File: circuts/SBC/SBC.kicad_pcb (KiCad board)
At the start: 2 copper layers, 141 parts, among them IC1 PIC16F15243-I_SS, J1 DE9_Plug, J10 Power, J2 OSTTC060162, J3 XT60-M, J4 OSTTC060162, J5 640456-3, J8 B5B-XH-A_LF__SN_, Q1 IRFS4227, Q10 MMBTA06, Q2 MMBTA06, Q3 MMBTA06, Q4 MMBTA06, Q5 MMBTA06, Q8 IRFS4227, Q9 MMBTA06, U1 3.3v, U2 UC3843, U3 BTS7960B, U5 LM358DT, U6 BTS7960B, U7 BTS7960B, U8 BTS7960B, U9 LM358DT

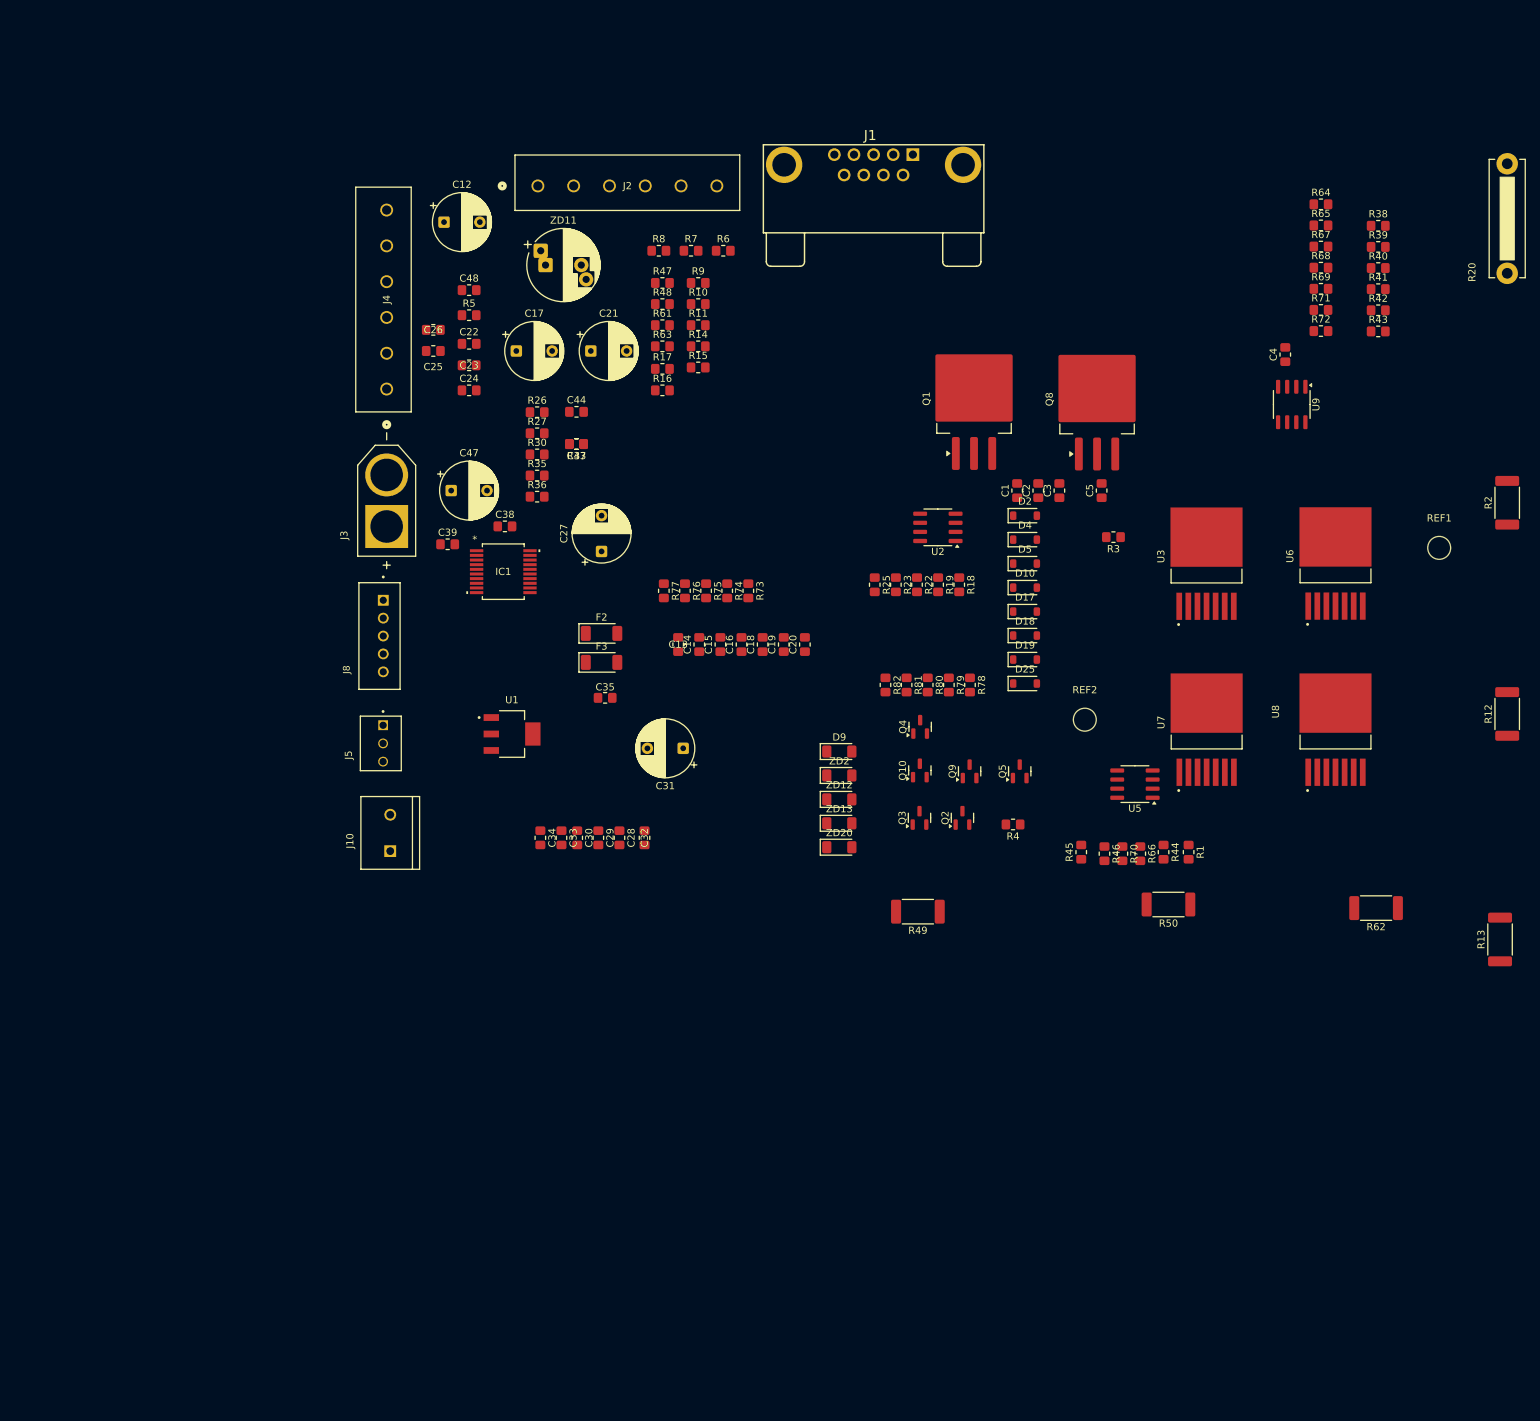
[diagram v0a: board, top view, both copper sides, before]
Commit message: layout
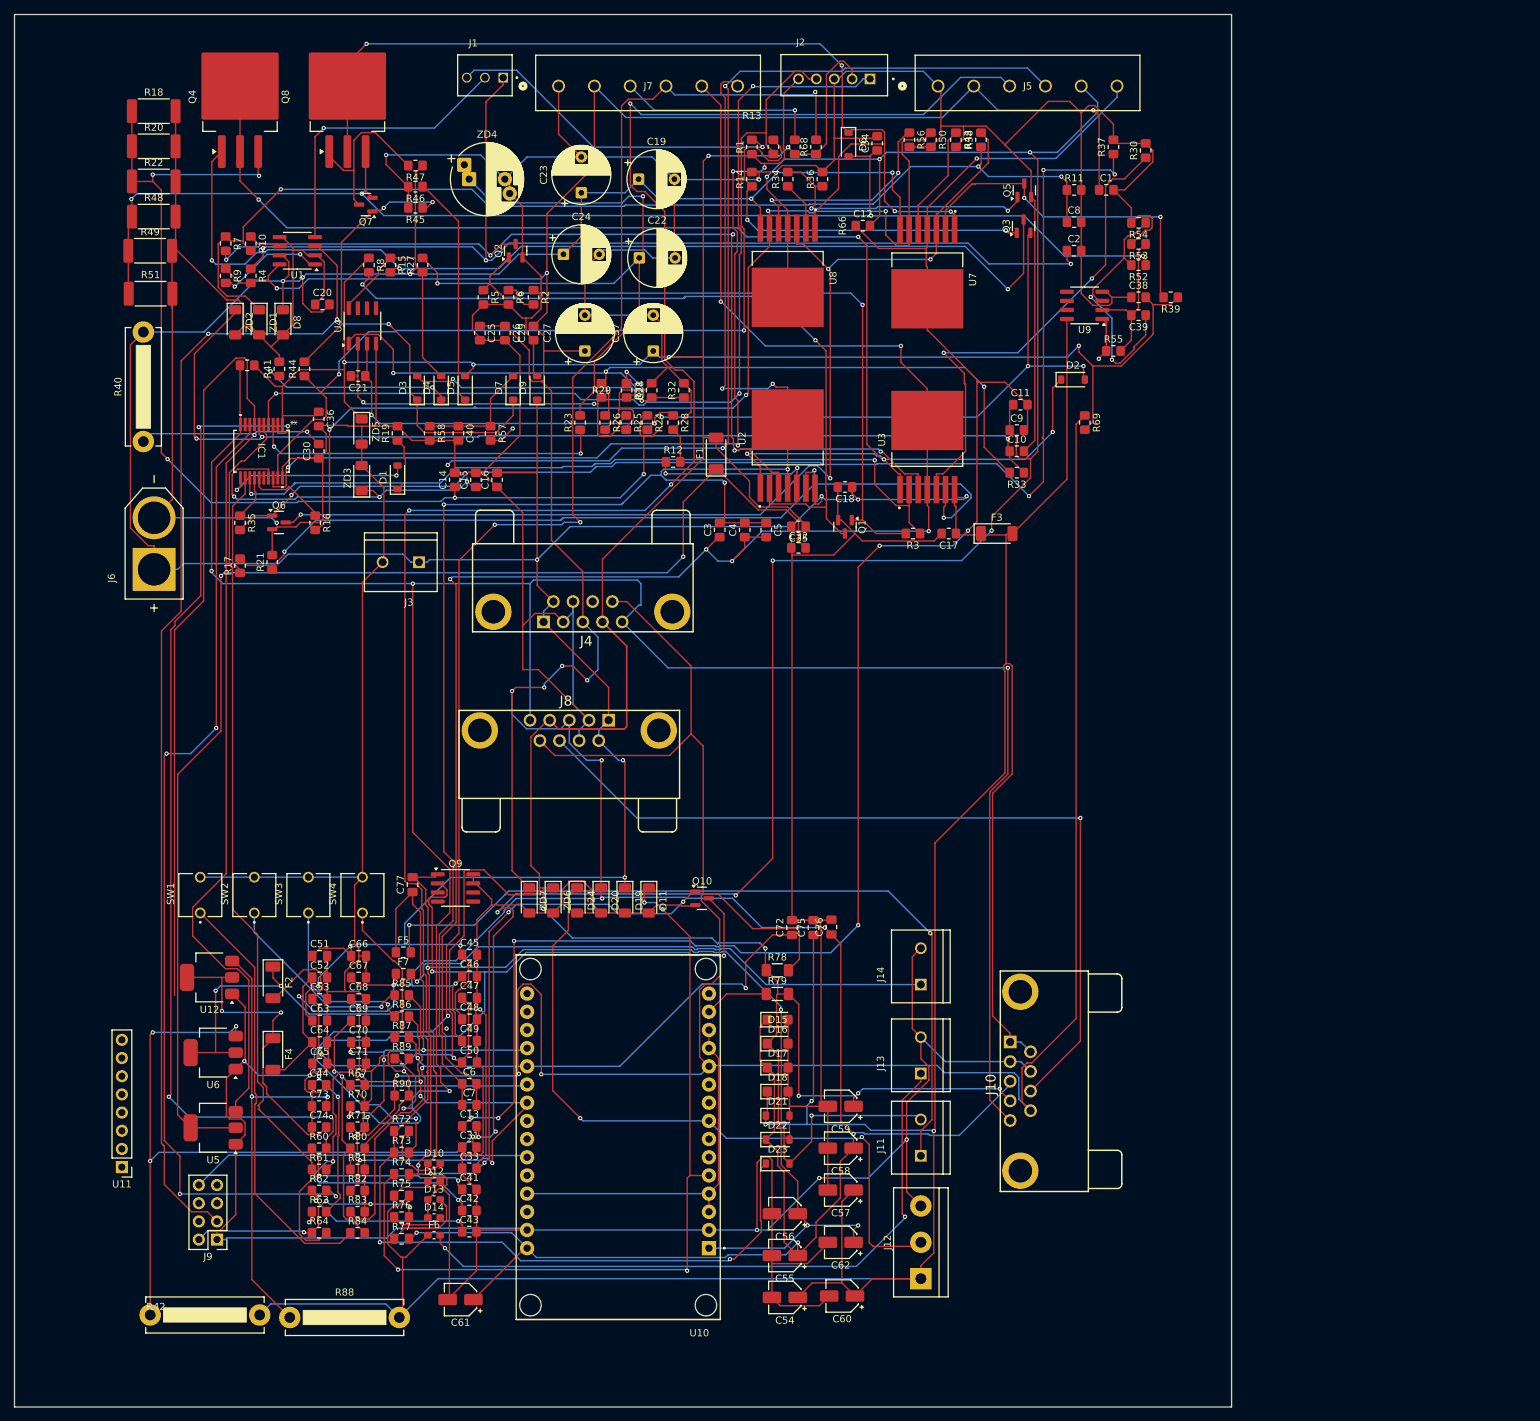
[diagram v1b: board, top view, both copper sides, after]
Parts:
- removed D25: 1N4004-T_NRND, Diode_SMD:D_SOD-123
- removed REF1, REF2: MountingHole_3.2mm_M3, MountingHole:MountingHole_3.2mm_M3
- removed ZD11: BZV55B4V7, Capacitor_THT:CP_Radial_D10.0mm_P5.00mm_P7.50mm
- removed ZD12, ZD13: BZV55B4V7, Diode_SMD:D_MiniMELF
- removed ZD20: 3.3v, Diode_SMD:D_MiniMELF
- added C10: 2uf, Resistor_SMD:R_0805_2012Metric_Pad1.20x1.40mm_HandSolder, F.Cu at (149.0, 77.0)
- added C11: 1nf, Resistor_SMD:R_0805_2012Metric_Pad1.20x1.40mm_HandSolder, F.Cu at (149.5, 70.5)
- added C36: 1nf, Resistor_SMD:R_0805_2012Metric_Pad1.20x1.40mm_HandSolder, F.Cu at (51.5, 72.5)
- added C37: 470uf, Capacitor_THT:CP_Radial_D8.0mm_P5.00mm, F.Cu at (98.2, 63.0)
- added C40: 2uf, Resistor_SMD:R_0805_2012Metric_Pad1.20x1.40mm_HandSolder, F.Cu at (71.0, 74.5)
- added C41: 1nf, Resistor_SMD:R_0805_2012Metric_Pad1.20x1.40mm_HandSolder, F.Cu at (72.5, 180.1)
- added C42: 1nf, Resistor_SMD:R_0805_2012Metric_Pad1.20x1.40mm_HandSolder, F.Cu at (72.5, 183.1)
- added C45: 1nf, Capacitor_SMD:C_0805_2012Metric_Pad1.18x1.45mm_HandSolder, F.Cu at (72.6, 147.3)
- added C46: 1nf, Capacitor_SMD:C_0805_2012Metric_Pad1.18x1.45mm_HandSolder, F.Cu at (72.6, 150.3)
- added C49: 100nf, Capacitor_SMD:C_0805_2012Metric_Pad1.18x1.45mm_HandSolder, F.Cu at (72.6, 159.4)
- added C50: 100nf, Capacitor_SMD:C_0805_2012Metric_Pad1.18x1.45mm_HandSolder, F.Cu at (72.6, 162.4)
- added C51: 2uf, Capacitor_SMD:C_0805_2012Metric_Pad1.18x1.45mm_HandSolder, F.Cu at (51.6, 147.5)
- added C52: 2uf, Capacitor_SMD:C_0805_2012Metric_Pad1.18x1.45mm_HandSolder, F.Cu at (51.6, 150.5)
- added C53: 2uf, Capacitor_SMD:C_0805_2012Metric_Pad1.18x1.45mm_HandSolder, F.Cu at (51.6, 153.5)
- added C54: 100uf, Capacitor_SMD:CP_Elec_4x4.5, F.Cu at (116.6, 195.2)
- added C55: 100uf, Capacitor_SMD:CP_Elec_4x4.5, F.Cu at (116.6, 189.3)
- added C56: 100uf, Capacitor_SMD:CP_Elec_4x4.5, F.Cu at (116.6, 183.5)
- added C57: 470uf, Capacitor_SMD:CP_Elec_4x4.5, F.Cu at (124.4, 180.2)
- added C58: 470uf, Capacitor_SMD:CP_Elec_4x4.5, F.Cu at (124.4, 174.3)
- added C59: 470uf, Capacitor_SMD:CP_Elec_4x4.5, F.Cu at (124.4, 168.5)
- added C6: 2uf, Resistor_SMD:R_0805_2012Metric_Pad1.20x1.40mm_HandSolder, F.Cu at (72.5, 165.4)
- added C60: 1000uf, Capacitor_SMD:CP_Elec_4x4.5, F.Cu at (124.6, 195.0)
- added C61: 1000uf, Capacitor_SMD:CP_Elec_4x4.5, F.Cu at (71.3, 195.5)
- added C62: 1000uf, Capacitor_SMD:CP_Elec_4x4.5, F.Cu at (124.4, 187.5)
- added C63: 2uf, Capacitor_SMD:C_0805_2012Metric_Pad1.18x1.45mm_HandSolder, F.Cu at (51.6, 156.5)
- added C64: 2uf, Capacitor_SMD:C_0805_2012Metric_Pad1.18x1.45mm_HandSolder, F.Cu at (51.6, 159.5)
- added C65: 2uf, Capacitor_SMD:C_0805_2012Metric_Pad1.18x1.45mm_HandSolder, F.Cu at (51.6, 162.5)
- added C66: 100nf, Capacitor_SMD:C_0805_2012Metric_Pad1.18x1.45mm_HandSolder, F.Cu at (57.1, 147.5)
- added C67: 100nf, Capacitor_SMD:C_0805_2012Metric_Pad1.18x1.45mm_HandSolder, F.Cu at (57.1, 150.5)
- added C68: 100nf, Capacitor_SMD:C_0805_2012Metric_Pad1.18x1.45mm_HandSolder, F.Cu at (57.1, 153.5)
- added C69: 100nf, Capacitor_SMD:C_0805_2012Metric_Pad1.18x1.45mm_HandSolder, F.Cu at (57.1, 156.5)
- added C7: 2uf, Resistor_SMD:R_0805_2012Metric_Pad1.20x1.40mm_HandSolder, F.Cu at (72.5, 168.3)
- added C70: 100nf, Capacitor_SMD:C_0805_2012Metric_Pad1.18x1.45mm_HandSolder, F.Cu at (57.1, 159.5)
- added C71: 100nf, Capacitor_SMD:C_0805_2012Metric_Pad1.18x1.45mm_HandSolder, F.Cu at (57.1, 162.6)
- added C72: 100nf, Capacitor_SMD:C_0805_2012Metric_Pad1.18x1.45mm_HandSolder, F.Cu at (117.6, 143.5)
- added C73: 100nf, Resistor_SMD:R_0805_2012Metric_Pad1.20x1.40mm_HandSolder, F.Cu at (51.5, 168.5)
- added C74: 100nf, Resistor_SMD:R_0805_2012Metric_Pad1.20x1.40mm_HandSolder, F.Cu at (51.5, 171.4)
- added C75: C, Capacitor_SMD:C_0805_2012Metric_Pad1.18x1.45mm_HandSolder, F.Cu at (120.6, 143.5)
- added C76: C, Capacitor_SMD:C_0805_2012Metric_Pad1.18x1.45mm_HandSolder, F.Cu at (123.1, 143.5)
- added C77: C, Capacitor_SMD:C_0805_2012Metric_Pad1.18x1.45mm_HandSolder, F.Cu at (64.6, 137.5)
- added C8: 100pf, Resistor_SMD:R_0805_2012Metric_Pad1.20x1.40mm_HandSolder, F.Cu at (157.0, 45.0)
- added C9: 100nf, Resistor_SMD:R_0805_2012Metric_Pad1.20x1.40mm_HandSolder, F.Cu at (149.0, 74.0)
- added D1: LED, Diode_SMD:D_SOD-123, F.Cu at (62.5, 80.7)
- added D11: BZV55B3V3, Diode_SMD:D_MiniMELF, F.Cu at (97.6, 139.8)
- added D12: LED, Capacitor_SMD:C_0603_1608Metric_Pad1.08x0.95mm_HandSolder, F.Cu at (67.6, 179.0)
- added D13: LED, Capacitor_SMD:C_0603_1608Metric_Pad1.08x0.95mm_HandSolder, F.Cu at (67.6, 181.5)
- added D14: LED, Capacitor_SMD:C_0603_1608Metric_Pad1.08x0.95mm_HandSolder, F.Cu at (67.6, 184.0)
- added D15: SMAJ6.5A, Diode_SMD:D_SMF, F.Cu at (115.6, 156.4)
- added D16: SMAJ6.5A, Diode_SMD:D_SMF, F.Cu at (115.6, 159.8)
- added D20: 5.6v zener, Diode_SMD:D_MiniMELF, F.Cu at (90.9, 139.8)
- added D21: 1N4004-T_NRND, Diode_SMD:D_SOD-123, F.Cu at (115.6, 169.8)
- added D22: 1N4004-T_NRND, Diode_SMD:D_SOD-123, F.Cu at (115.6, 173.2)
- added D23: 1N4004-T_NRND, Diode_SMD:D_SOD-123, F.Cu at (115.6, 176.5)
- added D24: BZV55B3V3, Diode_SMD:D_MiniMELF, F.Cu at (87.6, 139.8)
- added D3: 1N4004-T_NRND, Diode_SMD:D_SOD-123, F.Cu at (65.2, 68.2)
- added D6: 1N4004-T_NRND, Diode_SMD:D_SOD-123, F.Cu at (125.5, 34.1)
- added D7: 1N4004-T_NRND, Diode_SMD:D_SOD-123, F.Cu at (78.7, 68.2)
- added D8: 20v zener, Diode_SMD:D_MiniMELF, F.Cu at (46.5, 59.0)
- added F1: 1A, Diode_SMD:D_SOD-128, F.Cu at (107.0, 77.3)
- added F4: 1A, Diode_SMD:D_SOD-128, F.Cu at (45.1, 161.2)
- added F5: 1A, Capacitor_SMD:C_0805_2012Metric_Pad1.18x1.45mm_HandSolder, F.Cu at (63.3, 147.0)
- added F6: 1A, Capacitor_SMD:C_0603_1608Metric_Pad1.08x0.95mm_HandSolder, F.Cu at (67.6, 186.5)
- added F7: 1A, Capacitor_SMD:C_0805_2012Metric_Pad1.18x1.45mm_HandSolder, F.Cu at (63.3, 150.0)
- added J11: buzzer, 282837-2:TE_282837-2, F.Cu at (135.6, 172.9)
- added J12: metal detect, TerminalBlock:TerminalBlock_bornier-3_P5.08mm, F.Cu at (135.6, 192.6)
- added J13: 12v Power, 282837-2:TE_282837-2, F.Cu at (135.6, 161.4)
- added J14: 5v Power, 282837-2:TE_282837-2, F.Cu at (135.6, 149.0)
- added J6: XT60-M, XT60-M:AMASS_XT60-M, F.Cu at (28.5, 89.9)
- added J7: OSTTC060162, footprints:CONN_6P-OSTTC_OST, F.Cu at (85.0, 26.0)
- added J9: Conn_02x04_Odd_Even, Connector_PinHeader_2.54mm:PinHeader_2x04_P2.54mm_Vertical, F.Cu at (37.3, 187.1)
- added Q6: MMBTA06, Package_TO_SOT_SMD:SOT-23, F.Cu at (45.9, 87.0)
- added Q7: MMBTA06, Package_TO_SOT_SMD:SOT-23, F.Cu at (58.1, 42.5)
- added R21: 470, Resistor_SMD:R_0805_2012Metric_Pad1.20x1.40mm_HandSolder, F.Cu at (45.0, 92.5)
- added R24: 10k, Resistor_SMD:R_0805_2012Metric_Pad1.20x1.40mm_HandSolder, F.Cu at (97.4, 73.0)
- added R28: 56k, Resistor_SMD:R_0805_2012Metric_Pad1.20x1.40mm_HandSolder, F.Cu at (101.0, 73.0)
- added R29: 56k, Resistor_SMD:R_0805_2012Metric_Pad1.20x1.40mm_HandSolder, F.Cu at (91.0, 68.5)
- added R31: 100k, Resistor_SMD:R_0805_2012Metric_Pad1.20x1.40mm_HandSolder, F.Cu at (94.5, 68.5)
- added R32: 56k, Resistor_SMD:R_0805_2012Metric_Pad1.20x1.40mm_HandSolder, F.Cu at (102.5, 68.5)
- added R33: 2.2k, Resistor_SMD:R_0805_2012Metric_Pad1.20x1.40mm_HandSolder, F.Cu at (149.0, 80.0)
- added R34: 220, Resistor_SMD:R_0805_2012Metric_Pad1.20x1.40mm_HandSolder, F.Cu at (117.0, 39.0)
- added R51: 0.3, Resistor_SMD:R_2512_6332Metric_Pad1.40x3.35mm_HandSolder, F.Cu at (28.0, 55.0)
- added R52: 10k, Resistor_SMD:R_0805_2012Metric_Pad1.20x1.40mm_HandSolder, F.Cu at (166.0, 51.0)
- added R53: 10k, Resistor_SMD:R_0805_2012Metric_Pad1.20x1.40mm_HandSolder, F.Cu at (166.0, 48.0)
- added R54: 56k, Resistor_SMD:R_0805_2012Metric_Pad1.20x1.40mm_HandSolder, F.Cu at (166.0, 45.1)
- added R55: 56k, Resistor_SMD:R_0805_2012Metric_Pad1.20x1.40mm_HandSolder, F.Cu at (162.5, 63.0)
- added R56: 2k, Resistor_SMD:R_0805_2012Metric_Pad1.20x1.40mm_HandSolder, F.Cu at (134.0, 33.5)
- added R57: 100k, Resistor_SMD:R_0805_2012Metric_Pad1.20x1.40mm_HandSolder, F.Cu at (75.5, 74.5)
- added R58: 56k, Resistor_SMD:R_0805_2012Metric_Pad1.20x1.40mm_HandSolder, F.Cu at (67.0, 74.5)
- added R60: 5.1k, Resistor_SMD:R_0805_2012Metric_Pad1.20x1.40mm_HandSolder, F.Cu at (51.5, 174.4)
- added R83: 10k, Resistor_SMD:R_0805_2012Metric_Pad1.20x1.40mm_HandSolder, F.Cu at (56.9, 183.2)
- added R84: 1k, Resistor_SMD:R_0805_2012Metric_Pad1.20x1.40mm_HandSolder, F.Cu at (56.9, 186.2)
- added R85: 1k, Resistor_SMD:R_0805_2012Metric_Pad1.20x1.40mm_HandSolder, F.Cu at (63.1, 153.0)
- added R86: 1k, Resistor_SMD:R_0805_2012Metric_Pad1.20x1.40mm_HandSolder, F.Cu at (63.1, 155.9)
- added R87: 1k, Resistor_SMD:R_0805_2012Metric_Pad1.20x1.40mm_HandSolder, F.Cu at (63.1, 158.9)
- added R88: 200, Resistor_THT:R_Bare_Metal_Element_L16.3mm_W4.8mm_P15.30mm, F.Cu at (47.5, 198.0)
- added R89: 10k, Resistor_SMD:R_0805_2012Metric_Pad1.20x1.40mm_HandSolder, F.Cu at (63.1, 161.8)
- added R90: 10k, Resistor_SMD:R_0805_2012Metric_Pad1.20x1.40mm_HandSolder, F.Cu at (63.1, 167.0)
- added SW1: SW_Push, BUTT-2:SW_BUTT-2, F.Cu at (35.0, 139.0)
- added SW2: SW_Push, BUTT-2:SW_BUTT-2, F.Cu at (42.5, 139.0)
- added SW3: SW_Push, BUTT-2:SW_BUTT-2, F.Cu at (50.0, 139.0)
- added SW4: SW_Push, BUTT-2:SW_BUTT-2, F.Cu at (57.6, 139.0)
- added U10: ESP32-DEVKIT-V1, ESP32-DEVKIT-V1:MODULE_ESP32_DEVKIT_V1, F.Cu at (93.3, 172.8)
- added U11: ~, Connector_PinHeader_2.54mm:PinHeader_1x08_P2.54mm_Vertical, F.Cu at (24.0, 177.0)
- added U12: AMS1117-5.0, Package_TO_SOT_SMD:SOT-223-3_TabPin2, F.Cu at (36.2, 150.5)
- added U4: LM358DT, Package_SO:SOIC-8_3.9x4.9mm_P1.27mm, F.Cu at (57.6, 59.5)
- added ZD1: 3.3v, Diode_SMD:D_MiniMELF, F.Cu at (43.2, 59.0)
- added ZD3: BZV55B4V7, Diode_SMD:D_MiniMELF, F.Cu at (57.5, 80.8)
- added ZD4: BZV55B4V7, Capacitor_THT:CP_Radial_D10.0mm_P5.00mm_P7.50mm, F.Cu at (72.5, 39.0)
- added ZD5: BZV55B4V7, Diode_SMD:D_MiniMELF, F.Cu at (57.5, 74.2)
- added ZD6: BZV55B4V7, Diode_SMD:D_MiniMELF, F.Cu at (84.2, 139.8)
- added ZD7: BZV55B4V7, Diode_SMD:D_MiniMELF, F.Cu at (80.9, 139.8)
- C12: footprint Capacitor_THT:CP_Radial_D8.0mm_P5.00mm -> Resistor_SMD:R_0805_2012Metric_Pad1.20x1.40mm_HandSolder
- C15, C29, C34, C38: value 100nf -> 2uf
- C16, C20, C39: value 1nf -> 2uf
- C17, C31: value 470uf -> 100nf; footprint Capacitor_THT:CP_Radial_D8.0mm_P5.00mm -> Resistor_SMD:R_0805_2012Metric_Pad1.20x1.40mm_HandSolder
- C18, C2, C4, C43, C44: value 2uf -> 1nf
- C19: value 100nf -> 470uf; footprint Resistor_SMD:R_0805_2012Metric_Pad1.20x1.40mm_HandSolder -> Capacitor_THT:CP_Radial_D8.0mm_P5.00mm
- C21: value 470uf -> 2uf; footprint Capacitor_THT:CP_Radial_D8.0mm_P5.00mm -> Resistor_SMD:R_0805_2012Metric_Pad1.20x1.40mm_HandSolder
- C22: footprint Resistor_SMD:R_0805_2012Metric_Pad1.20x1.40mm_HandSolder -> Capacitor_THT:CP_Radial_D8.0mm_P5.00mm
- C23: value 100pf -> 470uf; footprint Resistor_SMD:R_0805_2012Metric_Pad1.20x1.40mm_HandSolder -> Capacitor_THT:CP_Radial_D8.0mm_P5.00mm
- C24: value 2uf -> 470uf; footprint Resistor_SMD:R_0805_2012Metric_Pad1.20x1.40mm_HandSolder -> Capacitor_THT:CP_Radial_D8.0mm_P5.00mm
- C3, C30: value 1nf -> 100nf
- C32, C35: value 2uf -> 100nf
- C47: value 470uf -> 1nf; footprint Capacitor_THT:CP_Radial_D8.0mm_P5.00mm -> Capacitor_SMD:C_0805_2012Metric_Pad1.18x1.45mm_HandSolder
- C48: value 2uf -> 100nf; footprint Resistor_SMD:R_0805_2012Metric_Pad1.20x1.40mm_HandSolder -> Capacitor_SMD:C_0805_2012Metric_Pad1.18x1.45mm_HandSolder
- D10: value 1N4004-T_NRND -> LED; footprint Diode_SMD:D_SOD-123 -> Capacitor_SMD:C_0603_1608Metric_Pad1.08x0.95mm_HandSolder
- D17, D18: value LED -> SMAJ6.5A; footprint Diode_SMD:D_SOD-123 -> Diode_SMD:D_SMF
- D19: value LED -> 20v zener; footprint Diode_SMD:D_SOD-123 -> Diode_SMD:D_MiniMELF
- D4, D5: value 1N4004-T_NRND -> LED
- D9: value 20v zener -> 1N4004-T_NRND; footprint Diode_SMD:D_MiniMELF -> Diode_SMD:D_SOD-123
- J1: value DE9_Plug -> 640456-3; footprint DB9:DB9 -> 640456-3:TE_640456-3
- J10: value Power -> motor_con; footprint 282837-2:TE_282837-2 -> DB9:DB9
- J2: value OSTTC060162 -> B5B-XH-A_LF__SN_; footprint footprints:CONN_6P-OSTTC_OST -> B5B-XH-A_LF__SN_:JST_B5B-XH-A_LF__SN_
- J3: value XT60-M -> Power; footprint XT60-M:AMASS_XT60-M -> 282837-2:TE_282837-2
- J4: value OSTTC060162 -> DE9_Plug; footprint footprints:CONN_6P-OSTTC_OST -> DB9:DB9
- J5: value 640456-3 -> OSTTC060162; footprint 640456-3:TE_640456-3 -> footprints:CONN_6P-OSTTC_OST
- J8: value B5B-XH-A_LF__SN_ -> grip_con; footprint B5B-XH-A_LF__SN_:JST_B5B-XH-A_LF__SN_ -> DB9:DB9
- Q1: value IRFS4227 -> MMBTA06; footprint Package_TO_SOT_SMD:TO-263-3_TabPin2 -> Package_TO_SOT_SMD:SOT-23
- Q10: value MMBTA06 -> BC817
- Q4: value MMBTA06 -> IRFS4227; footprint Package_TO_SOT_SMD:SOT-23 -> Package_TO_SOT_SMD:TO-263-3_TabPin2
- Q9: value MMBTA06 -> FDS4559; footprint Package_TO_SOT_SMD:SOT-23 -> Package_SO:SOIC-8_3.9x4.9mm_P1.27mm
- R1, R15, R17, R9: value 10k -> 2k
- R10: value 330 -> 10k
- R11: value 1.5k -> 3.3k
- R12: value 0.3 -> 2k; footprint Resistor_SMD:R_2512_6332Metric_Pad1.40x3.35mm_HandSolder -> Resistor_SMD:R_0805_2012Metric_Pad1.20x1.40mm_HandSolder
- R13, R2: value 0.3 -> 220; footprint Resistor_SMD:R_2512_6332Metric_Pad1.40x3.35mm_HandSolder -> Resistor_SMD:R_0805_2012Metric_Pad1.20x1.40mm_HandSolder
- R14: value 3.3k -> 5.1k
- R16, R43: value 470 -> 2k
- R18: value 26k -> 0.3; footprint Resistor_SMD:R_0805_2012Metric_Pad1.20x1.40mm_HandSolder -> Resistor_SMD:R_2512_6332Metric_Pad1.40x3.35mm_HandSolder
- R19: value 100k -> 330
- R20: value 200 -> 0.3; footprint Resistor_THT:R_Bare_Metal_Element_L16.3mm_W4.8mm_P15.30mm -> Resistor_SMD:R_2512_6332Metric_Pad1.40x3.35mm_HandSolder
- R22: value 220 -> 0.3; footprint Resistor_SMD:R_0805_2012Metric_Pad1.20x1.40mm_HandSolder -> Resistor_SMD:R_2512_6332Metric_Pad1.40x3.35mm_HandSolder
- R25, R71: value 220 -> 10k
- R26: value 2k -> 26k
- R27: value 10k -> 100k
- R3: value 56k -> 220
- R35: value 2k -> 220
- R36: value 2k -> 5.1k
- R37, R5, R6, R63: value 10k -> 5.1k
- R38: value 100k -> 2k
- R39, R65, R66, R69: value 56k -> 10k
- R4: value 2k -> 56k
- R40: value 470 -> 200; footprint Resistor_SMD:R_0805_2012Metric_Pad1.20x1.40mm_HandSolder -> Resistor_THT:R_Bare_Metal_Element_L16.3mm_W4.8mm_P15.30mm
- R41: value 2k -> 1.5k
- R42: value 2k -> 200; footprint Resistor_SMD:R_0805_2012Metric_Pad1.20x1.40mm_HandSolder -> Resistor_THT:R_Bare_Metal_Element_L16.3mm_W4.8mm_P15.30mm
- R44: value 56k -> 470
- R45: value 56k -> 5.1k
- R46: value 2.2k -> 330
- R48: value 330 -> 0.3; footprint Resistor_SMD:R_0805_2012Metric_Pad1.20x1.40mm_HandSolder -> Resistor_SMD:R_2512_6332Metric_Pad1.40x3.35mm_HandSolder
- R50: value 0.3 -> 470; footprint Resistor_SMD:R_2512_6332Metric_Pad1.40x3.35mm_HandSolder -> Resistor_SMD:R_0805_2012Metric_Pad1.20x1.40mm_HandSolder
- R61: value 470 -> 5.1k
- R62: value 0.3 -> 5.1k; footprint Resistor_SMD:R_2512_6332Metric_Pad1.40x3.35mm_HandSolder -> Resistor_SMD:R_0805_2012Metric_Pad1.20x1.40mm_HandSolder
- R67: value 2k -> 10k
- R68: value 100k -> 10k
- R7: value 10k -> 470
- R70: value 5k -> 10k
- R72: value 2k -> 1k; footprint Resistor_SMD:R_0805_2012Metric_Pad1.20x1.40mm_HandSolder -> Capacitor_SMD:C_0805_2012Metric_Pad1.18x1.45mm_HandSolder
- R73: value 10k -> 5k; footprint Resistor_SMD:R_0805_2012Metric_Pad1.20x1.40mm_HandSolder -> Capacitor_SMD:C_0805_2012Metric_Pad1.18x1.45mm_HandSolder
- R74, R75: value 220 -> 1k; footprint Resistor_SMD:R_0805_2012Metric_Pad1.20x1.40mm_HandSolder -> Capacitor_SMD:C_0805_2012Metric_Pad1.18x1.45mm_HandSolder
- R76: value 2k -> 220; footprint Resistor_SMD:R_0805_2012Metric_Pad1.20x1.40mm_HandSolder -> Capacitor_SMD:C_0805_2012Metric_Pad1.18x1.45mm_HandSolder
- R77: value 5.1k -> 330; footprint Resistor_SMD:R_0805_2012Metric_Pad1.20x1.40mm_HandSolder -> Capacitor_SMD:C_0805_2012Metric_Pad1.18x1.45mm_HandSolder
- R78, R79: value 5.1k -> 10k; footprint Resistor_SMD:R_0805_2012Metric_Pad1.20x1.40mm_HandSolder -> Resistor_SMD:R_1206_3216Metric_Pad1.30x1.75mm_HandSolder
- R80, R81, R82: value 5.1k -> 10k
- U1: value 3.3v -> UC3843; footprint REG1117-3.3:SOT230P700X180-4N -> Package_SO:SOIC-8_3.9x4.9mm_P1.27mm
- U2: value UC3843 -> BTS7960B; footprint Package_SO:SOIC-8_3.9x4.9mm_P1.27mm -> BTS7960B:DPAK127P1490X440-8N
- U5: value LM358DT -> AMS1117-3.3; footprint Package_SO:SOIC-8_3.9x4.9mm_P1.27mm -> Package_TO_SOT_SMD:SOT-223-3_TabPin2
- U6: value BTS7960B -> AMS1117-3.3; footprint BTS7960B:DPAK127P1490X440-8N -> Package_TO_SOT_SMD:SOT-223-3_TabPin2
- moved R42 221.6 mm to (27.9, 197.7)
- moved R64 200.5 mm to (51.5, 186.2)
- moved R20 189.9 mm to (28.4, 34.4), turned to 0 degrees
- moved R67 178.4 mm to (56.9, 165.5)
- moved R71 176.5 mm to (56.9, 171.4)
- moved R40 174.2 mm to (27.0, 75.7), turned to 90 degrees
- moved U6 171.0 mm to (36.8, 161.0), turned to 180 degrees
- moved R72 170.2 mm to (63.1, 171.9)
- moved R41 153.9 mm to (46.0, 65.5), turned to 90 degrees
- moved R62 152.8 mm to (51.5, 180.3), turned to 0 degrees
- moved R65 151.3 mm to (41.5, 65.0)
- moved R13 150.2 mm to (115.0, 34.5)
- moved R49 141.5 mm to (27.9, 49.0), turned to 0 degrees
- moved R2 139.0 mm to (81.5, 55.5), turned to -90 degrees
- moved R44 137.7 mm to (49.5, 65.5), turned to 90 degrees
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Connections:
- C1 pad 1: Net-(D4-A) -> 5v+
- C12 pad 1: Net-(ZD11-K) -> M1_R
- C12 pad 2: GND -> M1_L
- C13 pad 1: M1_current_sen -> M1_R
- C13 pad 2: GND -> M1_L
- C14 pad 1: M2_current_sen -> Net-(D2-A)
- C15 pad 1: 5v+ -> M1_current_sen
- C16 pad 1: 5v+ -> GND
- C16 pad 2: GND -> HV
- C17 pad 1: 5v+ -> HV
- C18 pad 1: GND -> HV
- C18 pad 2: 5v+ -> GND
- C2 pad 1: 5v+ -> Net-(C2-Pad1)
- C20 pad 1: HV -> GND
- C20 pad 2: GND -> HV
- C21 pad 1: HV -> Net-(C21-Pad1)
- C21 pad 2: GND -> Net-(C21-Pad2)
- C22 pad 1: GND -> Net-(ZD4-K)
- C22 pad 2: HV -> GND
- C23 pad 1: PWM -> HV
- C24 pad 1: Net-(C24-Pad1) -> HV
- C24 pad 2: Net-(C24-Pad2) -> GND
- C25 pad 1: M1_L -> 5v+
- C25 pad 2: M1_R -> GND
- C26 pad 1: M1_L -> 5v+
- C26 pad 2: M1_R -> GND
- C27 pad 1: HV -> 5v+
- C28 pad 1: M1_R -> Net-(D3-A)
- C28 pad 2: M1_L -> GND
- C29 pad 1: M2_L -> GND
- C29 pad 2: M2_R -> 5v+
- C3 pad 1: Net-(C3-Pad1) -> M2_L
- C3 pad 2: GND -> M2_R
- C30 pad 1: M2_L -> GND
- C30 pad 2: M2_R -> Net-(U5-VI)
- C31 pad 1: HV -> GND
- C31 pad 2: GND -> Net-(U6-VI)
- C32 pad 1: M2_R -> GND
- C32 pad 2: M2_L -> Net-(U5-VO)
- C33 pad 2: Net-(U1-OUT) -> Net-(U6-VO)
- C34 pad 1: GND -> Net-(D6-A)
- C34 pad 2: Net-(U1-IN) -> GND
- C35 pad 1: GND -> 3.3V
- C35 pad 2: HV -> GND
- C38 pad 1: 3.3V -> GND
- C38 pad 2: GND -> 3.3V
- C39 pad 1: 3.3V -> Net-(C39-Pad1)
- C39 pad 2: GND -> Net-(C39-Pad2)
- C4 pad 1: Net-(C4-Pad1) -> M2_L
- C4 pad 2: Net-(C4-Pad2) -> M2_R
- C43 pad 1: Net-(D25-A) -> Net-(C43-Pad1)
- C44 pad 1: Net-(D2-A) -> Net-(C44-Pad1)
- C48 pad 1: GND -> HV
- C48 pad 2: 3.3V -> GND
- C5 pad 1: Net-(D5-A) -> M2_R
- C5 pad 2: GND -> M2_L
- D10 pad 1: HV -> buzzing_gnd
- D10 pad 2: GND -> Net-(D10-A)
- D17 pad 1: Net-(D17-K) -> 5v+
- D17 pad 2: Motor2_OFF -> GND
- D18 pad 1: Net-(D18-K) -> HV
- D18 pad 2: 3.3v -> GND
- D19 pad 1: Net-(D19-K) -> HV
- D19 pad 2: HV -> GND
- D2 pad 1: CS -> Net-(D2-K)
- D4 pad 2: Net-(D4-A) -> HV
- D5 pad 1: CS -> Net-(D5-K)
- D5 pad 2: Net-(D5-A) -> 3.3v
- F2 pad 1: Net-(U1-OUT) -> Net-(U6-VO)
- F3 pad 2: HVblock -> HV
- J1 pad 1: HVblock -> Net-(C2-Pad1)
- J1 pad 2: GND -> Net-(U1-RC)
- J1 pad 3: 5v+ -> Net-(J1-Pad3)
- J10 pad 1: HVblock -> HV
- J2 pad 1: GND -> Mcler
- J2 pad 2: 5v+ -> 3.3V
- J2 pad 3: B2 -> GND
- J2 pad 4: A2 -> PGD
- J2 pad 5: M2_L -> PGC
- J4 pad 1: GND -> HV
- J4 pad 2: 5v+ -> GND
- J4 pad 3: B1 -> 5v+
- J4 pad 4: A1 -> 3.3V
- J4 pad 5: M1_L -> SCL
- J4 pad 6: M1_R -> HV
- J5 pad 1: Net-(C3-Pad1) -> GND
- J5 pad 2: Net-(U2-RC) -> 5v+
- J5 pad 3: Net-(J5-Pad3) -> Net-(C41-Pad1)
- J8 pad 1: Mcler -> HV
- J8 pad 2: 3.3V -> GND
- J8 pad 3: GND -> 5v+
- J8 pad 4: PGD -> 3.3V
- J8 pad 5: PGC -> SCL
- Q1 pad 1: Net-(Q1-G) -> Net-(Q1-B)
- Q1 pad 2: Net-(D25-K) -> GND
- Q1 pad 3: Net-(D25-A) -> M2_D1
- Q10 pad 3: INH1 -> Net-(Q10-C)
- Q2 pad 3: M2_D1 -> INH2
- Q3 pad 2: Net-(D25-A) -> Net-(D2-A)
- Q3 pad 3: Net-(Q1-G) -> Net-(Q3-C)
- Q4 pad 1: Net-(Q4-B) -> Net-(Q3-C)
- Q4 pad 2: GND -> Net-(D2-K)
- Q4 pad 3: INH2 -> Net-(D2-A)
- Q5 pad 2: Net-(D4-A) -> GND
- Q5 pad 3: Net-(Q5-C) -> M1_D1
- Q8 pad 1: Net-(Q5-C) -> Net-(Q7-C)
- Q8 pad 2: Net-(D4-K) -> Net-(D6-K)
- Q8 pad 3: Net-(D4-A) -> Net-(D6-A)
- Q9 pad 1: Net-(Q9-B) -> buzzing_gnd
- Q9 pad 2: GND -> Net-(Q10-C)
- Q9 pad 3: M1_D1 -> (no net)
- R1 pad 1: 3.3V -> PGC
- R1 pad 2: M2_D1 -> Net-(J1-Pad3)
- R10 pad 1: Net-(D18-K) -> Net-(U1-OUT)
- R10 pad 2: GND -> PWM
- R11 pad 1: Net-(D19-K) -> PWM
- R12 pad 1: Net-(D25-A) -> Net-(U2-SR)
- R13 pad 1: Net-(D25-A) -> PGD
- R13 pad 2: GND -> Net-(Q3-B)
- R14 pad 1: PWM -> Net-(Q3-B)
- R15 pad 1: Net-(U2-OUT) -> HV
- R15 pad 2: PWM -> Net-(Q3-C)
- R16 pad 1: PWM -> Net-(IC1-RC1)
- R16 pad 2: INH2 -> error 1
- R17 pad 1: SDA -> Net-(IC1-RB5)
- R17 pad 2: 3.3V -> error 2
- R18 pad 1: Net-(ZD11-K) -> Net-(D2-A)
- R19 pad 1: HV -> Net-(D1-K)
- R19 pad 2: Net-(ZD11-K) -> GND
- R2 pad 1: Net-(D25-A) -> Motor2_OFF
- R2 pad 2: GND -> Net-(Q2-B)
- R20 pad 1: Net-(U1-IN) -> Net-(D2-A)
- R20 pad 2: HV -> GND
- R22 pad 1: M2_S1 -> Net-(D2-A)
- R22 pad 2: Net-(Q2-B) -> GND
- R23 pad 1: Net-(D17-K) -> voltge_sen
- R23 pad 2: GND -> Net-(ZD4-K)
- R25 pad 1: PGD -> Net-(C21-Pad2)
- R25 pad 2: Net-(Q3-B) -> GND
- R26 pad 1: PGC -> Net-(ZD4-K)
- R26 pad 2: Net-(J5-Pad3) -> GND
- R27 pad 1: Net-(D25-A) -> HV
- R27 pad 2: Net-(C24-Pad1) -> Net-(ZD4-K)
- R3 pad 1: Net-(C3-Pad1) -> M2_S1
- R3 pad 2: 5v+ -> Net-(Q1-B)
- R35 pad 1: Net-(U7-SR) -> Motor1_OFF
- R35 pad 2: GND -> Net-(Q6-B)
- R36 pad 1: Net-(IC1-RB5) -> Net-(Q5-B)
- R36 pad 2: error 2 -> GND
- R37 pad 1: Net-(C24-Pad2) -> Net-(Q6-B)
- R38 pad 1: Net-(D2-A) -> PWM
- R38 pad 2: Net-(R38-Pad2) -> INH1
- R39 pad 1: Net-(D2-A) -> 3.3V
- R39 pad 2: GND -> M1_D1
- R4 pad 1: HV -> Net-(C2-Pad1)
- R4 pad 2: Net-(Q1-G) -> 5v+
- R40 pad 1: error 2 -> Net-(U5-VI)
- R40 pad 2: GND -> HV
- R41 pad 1: Net-(IC1-RC1) -> Net-(D4-K)
- R41 pad 2: error 1 -> GND
- R42 pad 1: Net-(U6-SR) -> Net-(U6-VI)
- R42 pad 2: GND -> HV
- R43 pad 1: PGD -> Net-(U7-SR)
- R43 pad 2: Net-(Q5-B) -> GND
- R44 pad 1: Net-(R38-Pad2) -> PGD
- R44 pad 2: Net-(C24-Pad2) -> Net-(Q7-B)
- R45 pad 1: Net-(C24-Pad1) -> Net-(Q7-B)
- R46 pad 1: M2_current_sen -> Net-(D5-K)
- R46 pad 2: Net-(R38-Pad2) -> GND
- R47 pad 2: Net-(Q5-C) -> Net-(Q7-C)
- R48 pad 1: voltge_sen -> Net-(D6-A)
- R48 pad 2: Net-(ZD11-K) -> GND
- R49 pad 1: Net-(D4-A) -> Net-(D6-A)
- R5 pad 1: 3.3V -> Net-(Q2-B)
- R5 pad 2: B1 -> GND
- R50 pad 1: Net-(D4-A) -> error 1
- R6 pad 1: 3.3V -> Net-(Q1-B)
- R6 pad 2: A1 -> GND
- R61 pad 1: error 1 -> A1
- R61 pad 2: GND -> Net-(C42-Pad1)
- R62 pad 1: Net-(D4-A) -> Net-(C43-Pad1)
- R62 pad 2: GND -> B2
- R63 pad 1: Net-(D4-A) -> A2
- R63 pad 2: Net-(C4-Pad1) -> Net-(C44-Pad1)
- R64 pad 1: Net-(C4-Pad2) -> 3.3V
- R64 pad 2: GND -> Net-(C41-Pad1)
- R65 pad 1: Net-(C4-Pad1) -> SCL
- R65 pad 2: GND -> 3.3V
- R66 pad 1: Net-(R66-Pad1) -> 3.3V
- R66 pad 2: Net-(C4-Pad2) -> Net-(C43-Pad1)
- R67 pad 1: Net-(U8-SR) -> 3.3V
- R67 pad 2: GND -> Net-(C42-Pad1)
- R68 pad 1: Net-(D5-A) -> 3.3V
- R68 pad 2: Net-(R66-Pad1) -> Net-(C44-Pad1)
- R69 pad 1: Net-(D5-A) -> SDA
- R69 pad 2: GND -> 3.3V
- R7 pad 1: 3.3V -> PWM
- R7 pad 2: B2 -> INH2
- R70 pad 1: M1_current_sen -> SCL
- R70 pad 2: Net-(R66-Pad1) -> 3.3V
- R71 pad 1: Motor2_OFF -> SDA
- R71 pad 2: Net-(Q4-B) -> 3.3V
- R72 pad 1: PWM -> 12v
- R72 pad 2: INH1 -> Net-(D10-A)
- R73 pad 1: 3.3V -> 12v
- R73 pad 2: M1_D1 -> Net-(Q10-C)
- R74 pad 1: Motor1_OFF -> buzz
- R75 pad 1: M1_S1 -> Net-(D12-A)
- R75 pad 2: Net-(Q9-B) -> HV
- R76 pad 1: 5v+ -> Net-(D14-A)
- R76 pad 2: Net-(U2-COMP) -> 3.3V
- R77 pad 1: Net-(Q3-B) -> Net-(D13-A)
- R77 pad 2: GND -> 5v+
- R78 pad 1: Net-(Q5-B) -> 3.3V
- R78 pad 2: GND -> SDA
- R79 pad 1: Net-(Q4-B) -> SDL
- R79 pad 2: GND -> 3.3V
- R8 pad 2: A2 -> M2_D1
- R80 pad 1: Net-(Q2-B) -> SW1
- R80 pad 2: GND -> 3.3V
- R81 pad 1: Net-(Q9-B) -> SW4
- R81 pad 2: GND -> 3.3V
- R82 pad 1: Net-(Q10-B) -> SW2
- R82 pad 2: GND -> 3.3V
- R9 pad 1: SCL -> 5v+
- R9 pad 2: 3.3V -> Net-(U1-COMP)
- U1 pad 1: Net-(U1-IN) -> Net-(U1-COMP)
- U1 pad 3: Net-(U1-OUT) -> CS
- U1 pad 4: (no net) -> Net-(U1-RC)
- U2 pad 1: Net-(U2-COMP) -> Net-(D2-K)
- U2 pad 2: GND -> M2_D1
- U2 pad 3: CS -> INH2
- U2 pad 4: Net-(U2-RC) -> M2_R
- U2 pad 5: GND -> Net-(U2-SR)
- U2 pad 6: Net-(U2-OUT) -> error 2
- U2 pad 8: 5v+ -> M2_R
- U3 pad 1: Net-(D25-K) -> Net-(D2-K)
- U3 pad 2: M2_D1 -> M2_S1
- U3 pad 4: M2_R -> M2_L
- U3 pad 8: M2_R -> M2_L
- U5 pad 1: Net-(R38-Pad2) -> GND
- U5 pad 2: Net-(C24-Pad2) -> Net-(U5-VO)
- U5 pad 3: Net-(C24-Pad1) -> Net-(U5-VI)
- U6 pad 1: Net-(D4-K) -> GND
- U6 pad 2: M1_D1 -> Net-(U6-VO)
- U6 pad 3: INH1 -> Net-(U6-VI)
- U7 pad 1: Net-(D25-K) -> Net-(D6-K)
- U7 pad 2: M2_S1 -> M1_D1
- U7 pad 3: INH2 -> INH1
- U7 pad 4: M2_L -> M1_R
- U7 pad 6: error 2 -> error 1
- U7 pad 8: M2_L -> M1_R
- U8 pad 1: Net-(D4-K) -> Net-(D6-K)
- U9 pad 1: Net-(R66-Pad1) -> Net-(R55-Pad1)
- U9 pad 2: Net-(C4-Pad2) -> Net-(C39-Pad2)
- U9 pad 3: Net-(C4-Pad1) -> Net-(C39-Pad1)
- ZD2 pad 1: 3.3V -> M2_current_sen
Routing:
- net GND: track 0.00 -> 1423.4 mm, vias 0 -> 8
- net HV: track 0.00 -> 951.2 mm, vias 0 -> 17
- net 3.3V: track 0.00 -> 716.9 mm, vias 0 -> 20
- net 5v+: track 0.00 -> 639.7 mm, vias 0 -> 16
- net SDA: track 0.00 -> 353.2 mm, vias 0 -> 3
- net SCL: track 0.00 -> 346.6 mm, vias 0 -> 6
- net M1_L: track 0.00 -> 302.9 mm, vias 0 -> 9
- net Net-(C41-Pad1): track 0.00 -> 289.4 mm, vias 0 -> 6
- net M1_R: track 0.00 -> 255.6 mm, vias 0 -> 7
- net M2_L: track 0.00 -> 244.0 mm, vias 0 -> 6
- net Net-(D2-A): track 0.00 -> 239.8 mm, vias 0 -> 8
- net M2_R: track 0.00 -> 228.1 mm, vias 0 -> 5
- net Net-(C44-Pad1): track 0.00 -> 227.7 mm, vias 0 -> 6
- net CS: track 0.00 -> 204.8 mm, vias 0 -> 3
- net Net-(D2-K): track 0.00 -> 198.8 mm, vias 0 -> 5
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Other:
- board outline added: 170 x 194.5 mm
